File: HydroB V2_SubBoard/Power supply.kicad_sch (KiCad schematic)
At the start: 17 parts, among them J11 Conn_01x02_Pin, J12 Conn_01x02_Pin, J2 12V, U4 LMR33620ADDA

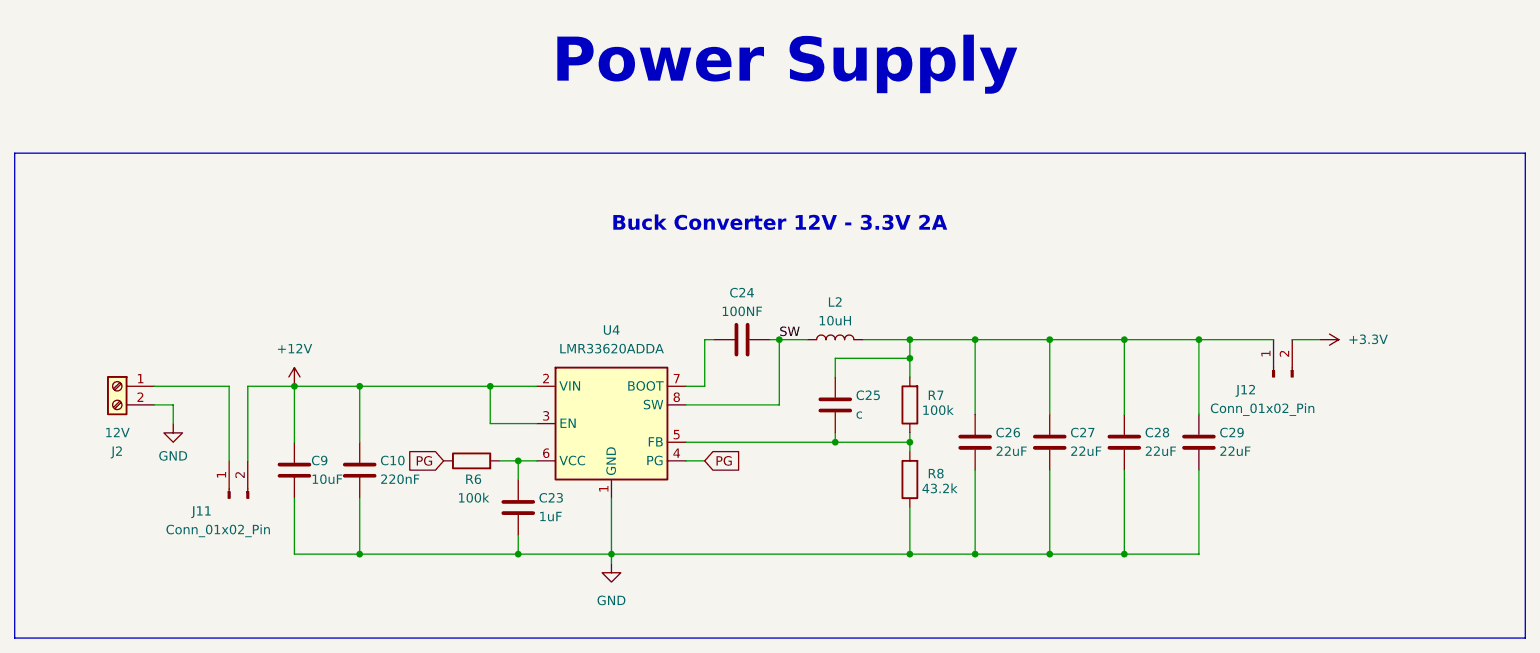
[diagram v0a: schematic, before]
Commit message: PCB layout
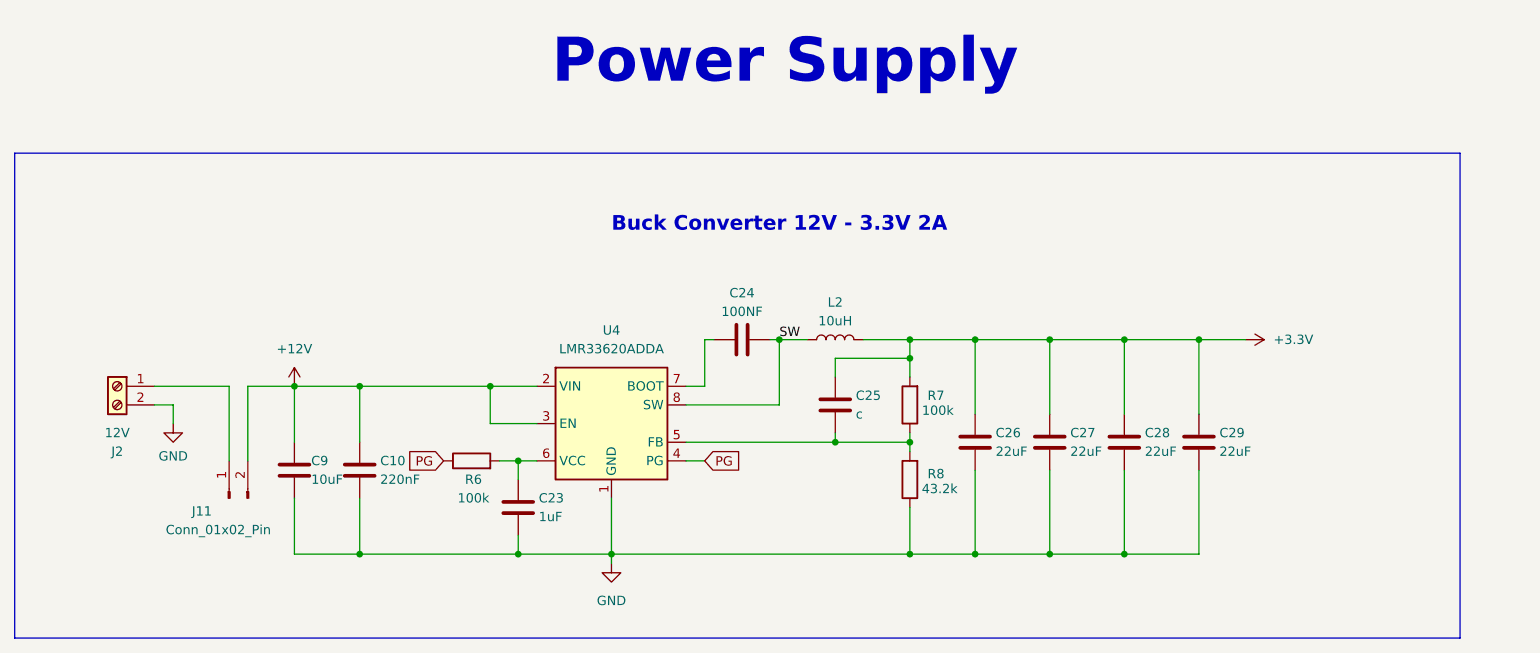
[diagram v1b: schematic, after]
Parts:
- removed J12: Conn_01x02_Pin, Connector_PinHeader_2.00mm:PinHeader_1x02_P2.00mm_Vertical, symbol Connector:Conn_01x02_Pin
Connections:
- net +3.3V: now also C25.1, C26.1, C27.1, C28.1, C29.1, L2.2, R7.2
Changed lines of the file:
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@@
-	(wire
-		(pts
-			(xy 220.98 100.33) (xy 224.79 100.33)
-		)
-		(stroke
-			(width 0)
-			(type default)
-		)
-	)
 	(wire
 		(pts
@@
 	(wire
 		(pts
-			(xy 208.28 100.33) (xy 218.44 100.33)
+			(xy 208.28 100.33) (xy 214.63 100.33)
 		)
 		(stroke
@@
 	(rectangle
 		(start 46.99 74.93)
-		(end 252.73 140.97)
+		(end 243.84 140.97)
 		(stroke
 			(width 0)
@@
 	(symbol
 		(lib_id "power:+3.3V")
-		(at 224.79 100.33 270)
+		(at 214.63 100.33 270)
 		(unit 1)
 		(exclude_from_sim no)
@@
 		(fields_autoplaced yes)
 		(property "Reference" "#PWR021"
-			(at 220.98 100.33 0)
+			(at 210.82 100.33 0)
 			(effects
 				(font
@@
 		)
 		(property "Value" "+3.3V"
-			(at 228.6 100.3299 90)
+			(at 218.44 100.3299 90)
 			(effects
 				(font
@@
 		)
 		(property "Footprint" ""
-			(at 224.79 100.33 0)
+			(at 214.63 100.33 0)
 			(effects
 				(font
@@
 		)
 		(property "Datasheet" ""
-			(at 224.79 100.33 0)
+			(at 214.63 100.33 0)
 			(effects
 				(font
@@
 		)
 		(property "Description" "Power symbol creates a global label with name \"+3.3V\""
-			(at 224.79 100.33 0)
+			(at 214.63 100.33 0)
 			(effects
 				(font
@@
 					(unit 1)
 				)
-			)
-		)
-	)
-	(symbol
-		(lib_id "Connector:Conn_01x02_Pin")
-		(at 218.44 105.41 90)
-		(unit 1)
-		(exclude_from_sim no)
-		(in_bom yes)
-		(on_board yes)
-		(dnp no)
-		(property "Reference" "J12"
-			(at 213.36 107.188 90)
-			(effects
-				(font
-					(size 1.27 1.27)
-				)
-				(justify right)
-			)
-		)
-		(property "Value" "Conn_01x02_Pin"
-			(at 209.804 109.728 90)
-			(effects
-				(font
-					(size 1.27 1.27)
-				)
-				(justify right)
-			)
-		)
-		(property "Footprint" "Connector_PinHeader_2.00mm:PinHeader_1x02_P2.00mm_Vertical"
-			(at 218.44 105.41 0)
-			(effects
-				(font
-					(size 1.27 1.27)
-				)
-				(hide yes)
-			)
-		)
-		(property "Datasheet" "~"
-			(at 218.44 105.41 0)
-			(effects
-				(font
-					(size 1.27 1.27)
-				)
-				(hide yes)
-			)
-		)
-		(property "Description" "Generic connector, single row, 01x02, script generated"
-			(at 218.44 105.41 0)
-			(effects
-				(font
-					(size 1.27 1.27)
-				)
-				(hide yes)
-			)
-		)
-		(pin "2"
-		)
-		(pin "1"
-		)
-		(instances
-			(project "HydroB V2"
-				(path "/0a8bb8df-6bdd-4d10-933b-144d3fa4f517/b5cea501-254b-4c6a-af47-d8c013c279ab/d50825f3-7645-4f22-8c9c-6a6002c3efba"
-					(reference "J12")
-					(unit 1)
-				)
